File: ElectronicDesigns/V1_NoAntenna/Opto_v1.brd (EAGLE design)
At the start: 100 x 80 mm, 7 parts

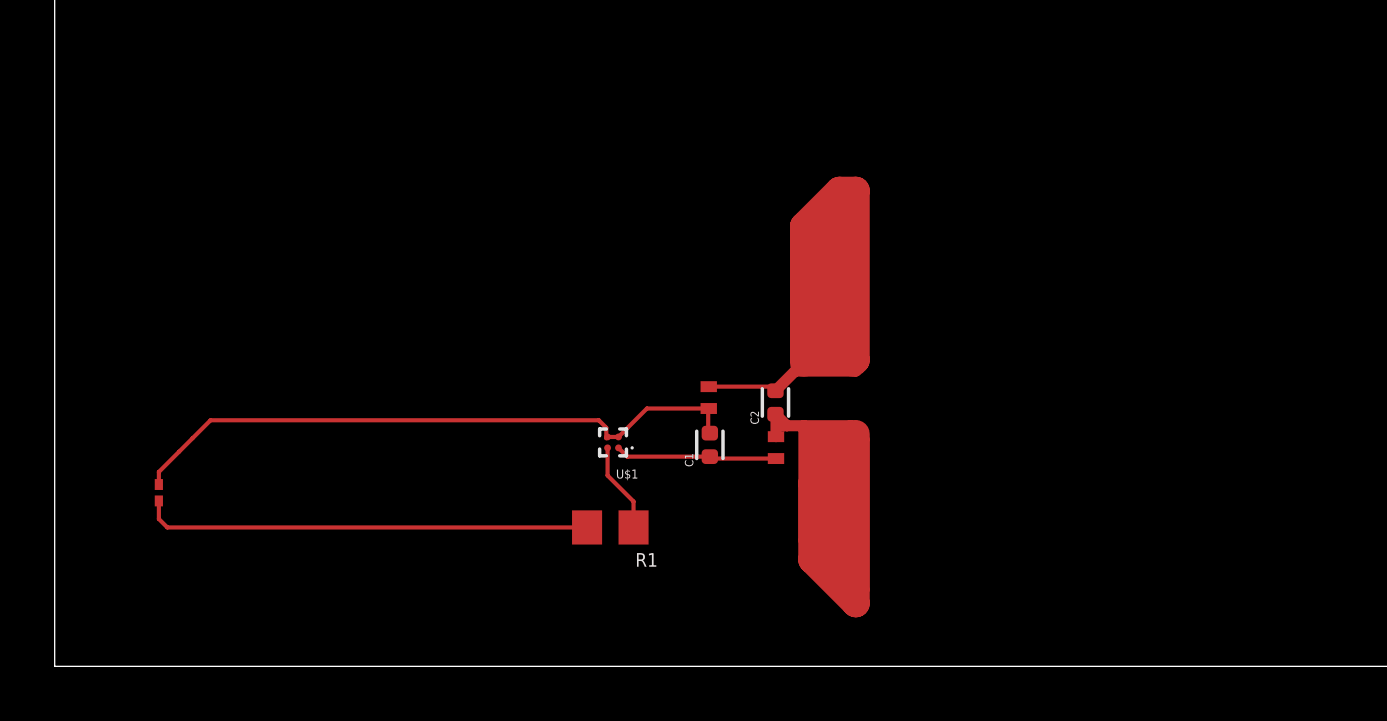
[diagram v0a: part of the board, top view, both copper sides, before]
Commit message: Update gerbers
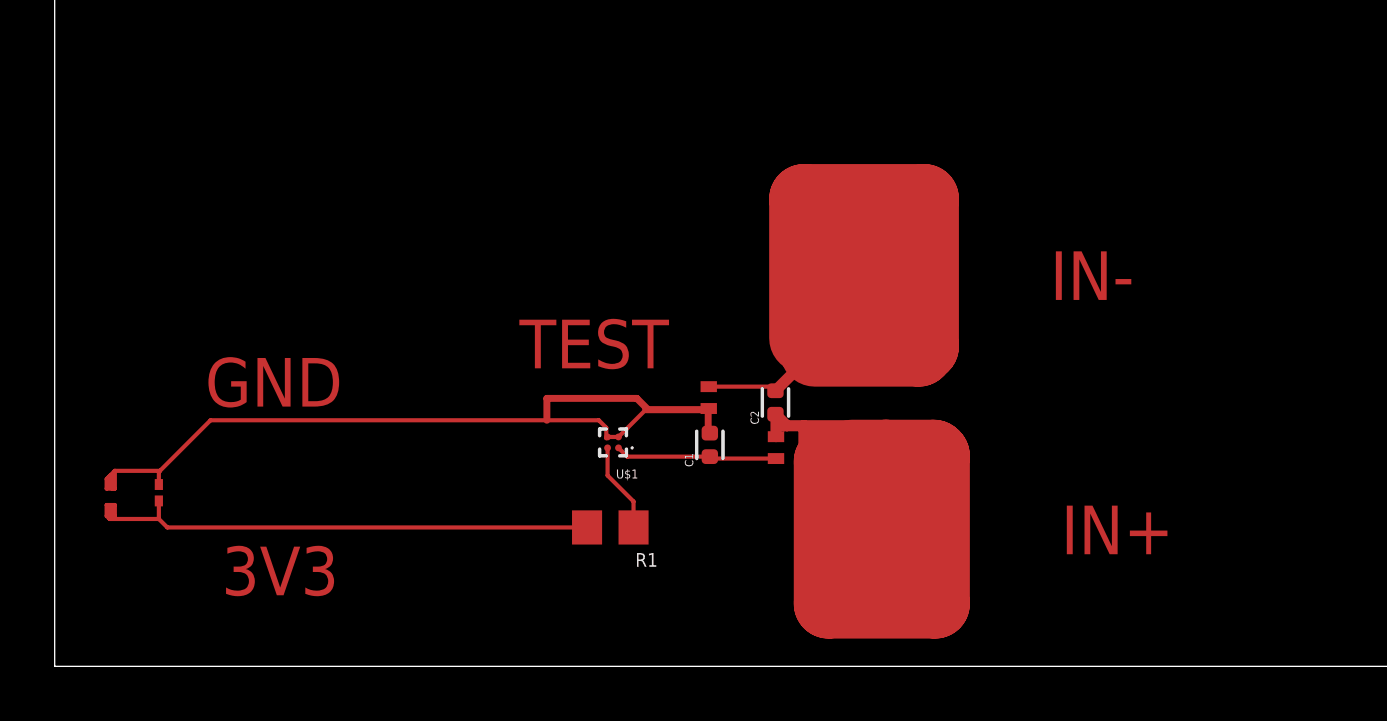
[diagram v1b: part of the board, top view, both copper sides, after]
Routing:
- net IN-: track 47.6 -> 70.3 mm
- net IN+: track 45.7 -> 67.4 mm
- net GND: track 23.2 -> 35.0 mm
- net N$2: track 16.4 -> 20.5 mm
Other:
- board text added: "3V3"
- board text added: "GND"
- board text added: "IN+"
- board text added: "IN-"
- board text added: "TEST"
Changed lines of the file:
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@@
 <wire x1="100" y1="80" x2="0" y2="80" width="0" layer="20"/>
 <wire x1="0" y1="80" x2="0" y2="0" width="0" layer="20"/>
+<text x="17" y="10.9" size="1.778" layer="1">TEST</text>
+<text x="36.8" y="4.1" size="1.778" layer="1">IN+</text>
+<text x="36.4" y="13.4" size="1.778" layer="1">IN-</text>
+<text x="5.5" y="9.5" size="1.778" layer="1">GND</text>
+<text x="6.1" y="2.6" size="1.778" layer="1">3V3</text>
 </plain>
 <attributes>
@@
 <wire x1="27.9" y1="8.2" x2="27.9" y2="4.1" width="1.016" layer="1"/>
 <wire x1="27.9" y1="4.1" x2="29.1" y2="2.9" width="1.016" layer="1"/>
-<wire x1="28.5" y1="4.3" x2="28.5" y2="7.5" width="1.016" layer="1"/>
+<wire x1="28.5" y1="4.3" x2="28.5" y2="5.6" width="1.016" layer="1"/>
 <wire x1="28.5" y1="7.5" x2="28.6" y2="7.6" width="1.016" layer="1"/>
 <wire x1="28.5" y1="7.5" x2="27.7" y2="6.7" width="1.016" layer="1"/>
@@
 <wire x1="27.7" y1="3.9" x2="29.3" y2="2.3" width="1.016" layer="1"/>
 <wire x1="29.3" y1="2.3" x2="29.3" y2="8.5" width="1.016" layer="1"/>
-<wire x1="27.7" y1="3.9" x2="27.9" y2="4.1" width="0" layer="19" extent="1-1"/>
+<wire x1="28.5" y1="5.6" x2="28.5" y2="7.5" width="2.54" layer="1"/>
+<wire x1="29.15" y1="7.75" x2="30.4" y2="7.75" width="2.54" layer="1"/>
+<wire x1="30.4" y1="7.75" x2="32.15" y2="7.75" width="2.54" layer="1"/>
+<wire x1="32.15" y1="7.75" x2="32.2" y2="7.7" width="2.54" layer="1"/>
+<wire x1="32.2" y1="7.7" x2="32.2" y2="2.286" width="2.54" layer="1"/>
+<wire x1="32.2" y1="2.286" x2="28.3" y2="2.286" width="2.54" layer="1"/>
+<wire x1="28.3" y1="2.286" x2="28.3" y2="7.5" width="2.54" layer="1"/>
+<wire x1="28.3" y1="7.5" x2="28.5" y2="7.5" width="2.54" layer="1"/>
+<wire x1="30.4" y1="7.75" x2="30.4" y2="3.8" width="2.54" layer="1"/>
 </signal>
 <signal name="IN-">
@@
 <wire x1="26.36" y1="10.08" x2="27.08" y2="10.8" width="0.4064" layer="1"/>
 <wire x1="27.08" y1="10.8" x2="29.3" y2="10.8" width="0.4064" layer="1"/>
-<wire x1="29.3" y1="10.8" x2="29.3" y2="14.3" width="0.4064" layer="1"/>
+<wire x1="29.3" y1="10.8" x2="29.3" y2="12.3" width="0.4064" layer="1"/>
+<wire x1="29.3" y1="12.3" x2="29.3" y2="14.3" width="0.4064" layer="1"/>
 <wire x1="29.3" y1="14.3" x2="29.1" y2="14.5" width="0.4064" layer="1"/>
 <wire x1="29.1" y1="14.5" x2="29.1" y2="13.8" width="1.27" layer="1"/>
@@
 <wire x1="27.7" y1="11.3" x2="27.6" y2="11.4" width="1.27" layer="1"/>
 <wire x1="29.1" y1="16.2" x2="29.1" y2="11.3" width="1.27" layer="1"/>
-<wire x1="27.4" y1="11.1" x2="27.4" y2="16.1" width="1.016" layer="1"/>
+<wire x1="27.4" y1="11.1" x2="27.4" y2="12" width="1.016" layer="1"/>
+<wire x1="27.4" y1="12" x2="27.4" y2="16.1" width="1.016" layer="1"/>
 <wire x1="27.4" y1="16.1" x2="28.7" y2="17.4" width="1.016" layer="1"/>
 <wire x1="28.7" y1="17.4" x2="29.3" y2="17.4" width="1.016" layer="1"/>
-<wire x1="29.3" y1="17.4" x2="29.3" y2="11.2" width="1.016" layer="1"/>
+<wire x1="29.3" y1="17.4" x2="29.3" y2="12.3" width="1.016" layer="1"/>
+<wire x1="29.3" y1="12.3" x2="29.3" y2="11.2" width="1.016" layer="1"/>
 <wire x1="29.3" y1="11.2" x2="29.2" y2="11.1" width="1.016" layer="1"/>
-<wire x1="29.1" y1="11.3" x2="29.3" y2="11.2" width="0" layer="19" extent="1-1"/>
+<wire x1="27.4" y1="12" x2="27.4" y2="17.1" width="2.54" layer="1"/>
+<wire x1="27.4" y1="17.1" x2="31.8" y2="17.1" width="2.54" layer="1"/>
+<wire x1="31.8" y1="17.1" x2="31.8" y2="11.7" width="2.54" layer="1"/>
+<wire x1="31.8" y1="11.7" x2="31.6" y2="11.5" width="2.54" layer="1"/>
+<wire x1="31.6" y1="11.5" x2="27.8" y2="11.5" width="2.54" layer="1"/>
+<wire x1="29.3" y1="12.3" x2="30.2" y2="13.2" width="2.54" layer="1"/>
+<wire x1="30.2" y1="13.2" x2="30.2" y2="15.7" width="2.54" layer="1"/>
 </signal>
 <signal name="N$4">
@@
 <wire x1="3.81" y1="6.65" x2="3.81" y2="7.11" width="0.1524" layer="1"/>
 <wire x1="20.22" y1="8.39" x2="20.1736" y2="8.3436" width="0.1524" layer="1"/>
-<wire x1="3.81" y1="7.11" x2="4.55" y2="7.85" width="0.1524" layer="1"/>
-<wire x1="4.55" y1="7.85" x2="5.0436" y2="8.3436" width="0.1524" layer="1"/>
-<wire x1="20.62" y1="8.39" x2="21.66" y2="9.43" width="0.1524" layer="1"/>
+<wire x1="20.62" y1="8.39" x2="21.615" y2="9.385" width="0.1524" layer="1"/>
+<wire x1="21.615" y1="9.385" x2="21.66" y2="9.43" width="0.1524" layer="1"/>
 <wire x1="21.66" y1="9.43" x2="23.9" y2="9.43" width="0.1524" layer="1"/>
 <wire x1="23.9" y1="9.43" x2="23.92" y2="9.43" width="0.1524" layer="1"/>
@@
 <wire x1="20.1736" y1="8.3436" x2="20.1736" y2="8.7264" width="0.1524" layer="1"/>
 <wire x1="20.1736" y1="8.7264" x2="19.9" y2="9" width="0.1524" layer="1"/>
-<wire x1="5.7" y1="9" x2="5.0436" y2="8.3436" width="0.1524" layer="1"/>
-<wire x1="19.9" y1="9" x2="5.7" y2="9" width="0.1524" layer="1"/>
+<wire x1="5.7" y1="9" x2="3.85" y2="7.15" width="0.1524" layer="1"/>
+<wire x1="3.85" y1="7.15" x2="3.81" y2="7.11" width="0.1524" layer="1"/>
+<wire x1="19.9" y1="9" x2="18" y2="9" width="0.1524" layer="1"/>
+<wire x1="18" y1="9" x2="5.7" y2="9" width="0.1524" layer="1"/>
+<wire x1="23.92" y1="9.43" x2="23.9" y2="9.41" width="0.254" layer="1"/>
+<wire x1="23.9" y1="9.41" x2="23.9" y2="8.59" width="0.254" layer="1"/>
+<wire x1="23.92" y1="9.43" x2="23.875" y2="9.385" width="0.254" layer="1"/>
+<wire x1="23.875" y1="9.385" x2="21.615" y2="9.385" width="0.254" layer="1"/>
+<wire x1="18" y1="9" x2="18" y2="9.8" width="0.254" layer="1"/>
+<wire x1="18" y1="9.8" x2="21.29" y2="9.8" width="0.254" layer="1"/>
+<wire x1="21.29" y1="9.8" x2="21.66" y2="9.43" width="0.254" layer="1"/>
+<wire x1="3.85" y1="7.15" x2="2.2" y2="7.15" width="0.1524" layer="1"/>
+<wire x1="2.2" y1="7.15" x2="2.2" y2="6.5" width="0.1524" layer="1"/>
+<wire x1="2.2" y1="6.5" x2="2.1" y2="6.5" width="0.1524" layer="1"/>
+<wire x1="2.1" y1="6.5" x2="1.9" y2="6.5" width="0.1524" layer="1"/>
+<wire x1="1.9" y1="6.5" x2="1.9" y2="6.85" width="0.1524" layer="1"/>
+<wire x1="1.9" y1="6.85" x2="1.975" y2="6.925" width="0.1524" layer="1"/>
+<wire x1="1.975" y1="6.925" x2="2.025" y2="6.975" width="0.1524" layer="1"/>
+<wire x1="2.025" y1="6.975" x2="2.2" y2="7.15" width="0.1524" layer="1"/>
+<wire x1="2.1" y1="6.6" x2="2.1" y2="6.9" width="0.1524" layer="1"/>
+<wire x1="2.1" y1="6.9" x2="2" y2="6.8" width="0.1524" layer="1"/>
+<wire x1="2" y1="6.8" x2="2" y2="6.6" width="0.1524" layer="1"/>
+<wire x1="2.1" y1="6.6" x2="2.1" y2="6.5" width="0" layer="19" extent="1-1"/>
 </signal>
 <signal name="N$1">
@@
 <wire x1="19.47" y1="5.08" x2="4.12" y2="5.08" width="0.1524" layer="1"/>
 <wire x1="4.12" y1="5.08" x2="3.81" y2="5.39" width="0.1524" layer="1"/>
+<wire x1="3.81" y1="5.39" x2="2.01" y2="5.39" width="0.1524" layer="1"/>
+<wire x1="1.9" y1="5.9" x2="2.2" y2="5.9" width="0.1524" layer="1"/>
+<wire x1="2.2" y1="5.5" x2="2" y2="5.5" width="0.1524" layer="1"/>
+<wire x1="2" y1="5.5" x2="2" y2="5.7" width="0.1524" layer="1"/>
+<wire x1="2" y1="5.7" x2="2.1" y2="5.8" width="0.1524" layer="1"/>
+<wire x1="2.1" y1="5.8" x2="2" y2="5.8" width="0.1524" layer="1"/>
+<wire x1="2" y1="5.8" x2="2" y2="5.7" width="0.1524" layer="1"/>
+<wire x1="2" y1="5.7" x2="2.1" y2="5.6" width="0.1524" layer="1"/>
+<wire x1="2.1" y1="5.6" x2="2.1" y2="5.7" width="0.1524" layer="1"/>
+<wire x1="2.01" y1="5.39" x2="1.9" y2="5.5" width="0.1524" layer="1"/>
+<wire x1="1.9" y1="5.5" x2="1.9" y2="5.9" width="0.1524" layer="1"/>
+<wire x1="2.2" y1="5.9" x2="2.2" y2="5.5" width="0.1524" layer="1"/>
 </signal>
 </signals>
